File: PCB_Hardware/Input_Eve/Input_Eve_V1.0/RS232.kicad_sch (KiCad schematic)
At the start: 10 parts, among them U9 MAX3232

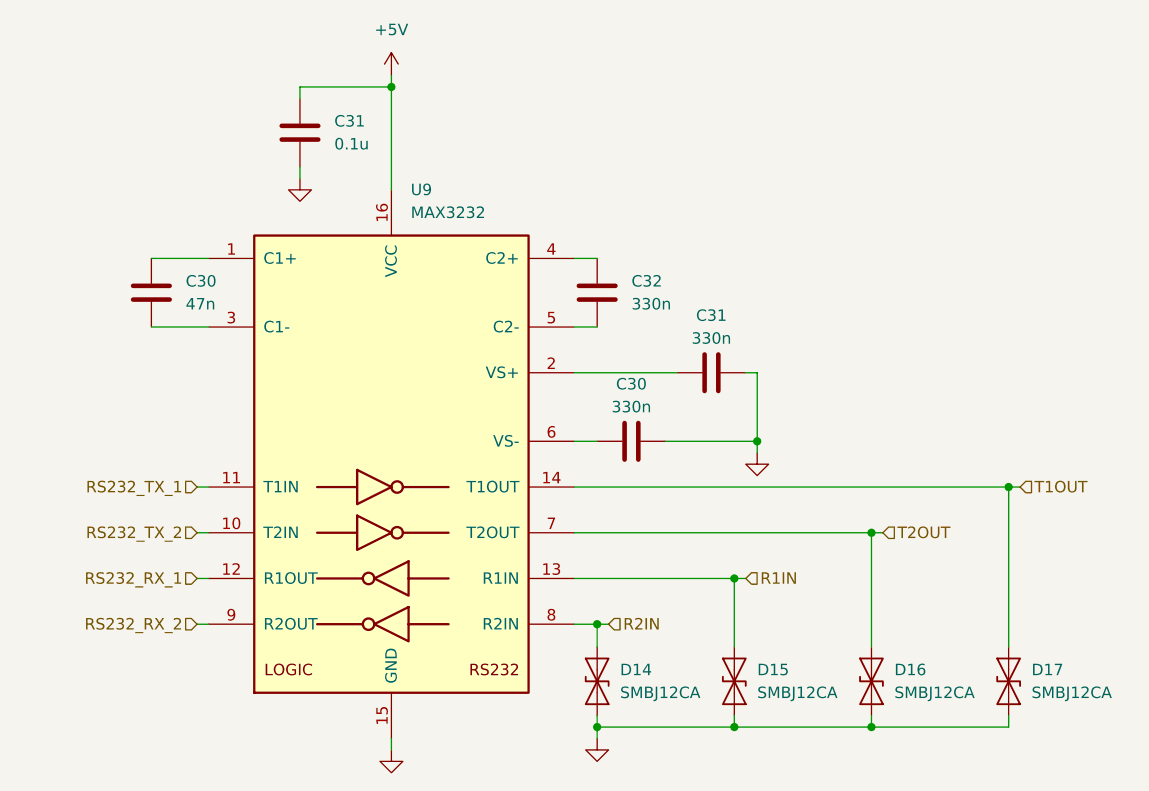
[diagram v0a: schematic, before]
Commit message: Update w new boards/firmware
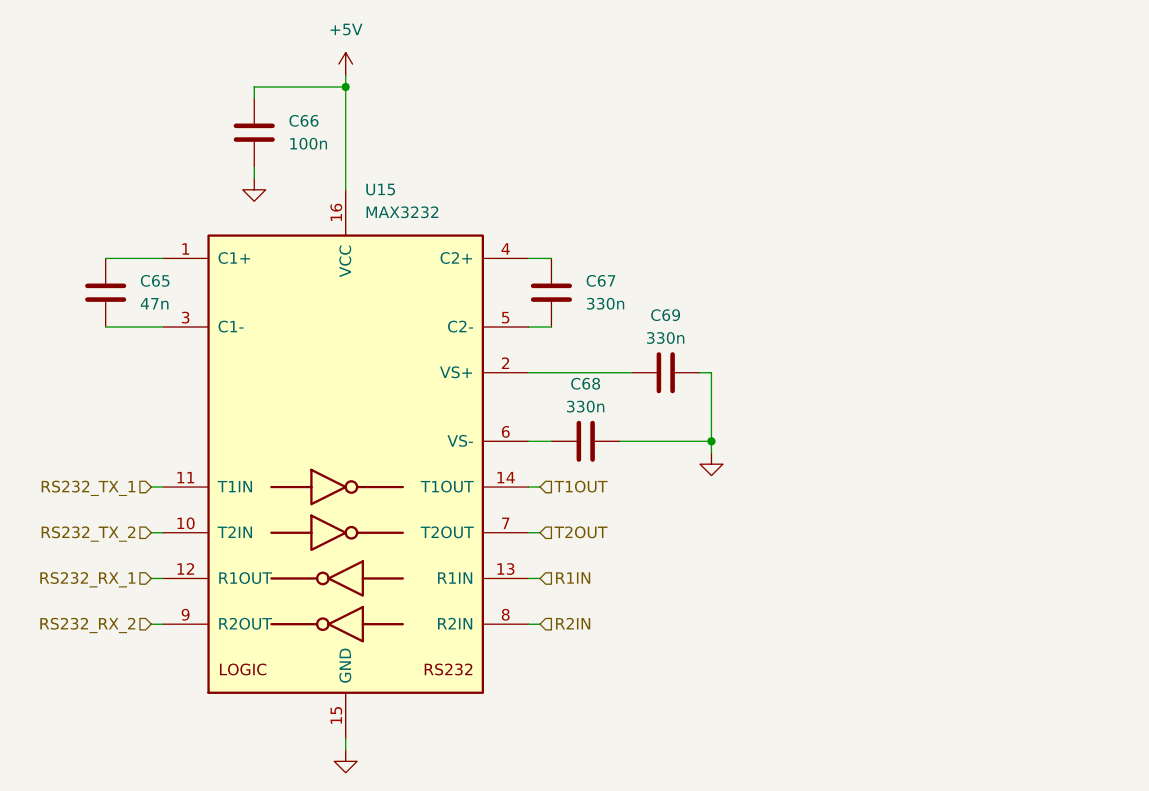
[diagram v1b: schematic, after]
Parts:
- removed C30: 47n, Capacitor_SMD:C_0402_1005Metric, symbol Device:C
- removed C30, C31, C32: 330n, Capacitor_SMD:C_0402_1005Metric, symbol Device:C
- removed C31: 0.1u, Capacitor_SMD:C_0402_1005Metric, symbol Device:C
- removed D14, D15, D16, D17: SMBJ12CA, Diode_SMD:D_SMA, symbol Diode:SMAJ6.0CA
- removed U9: MAX3232, symbol Interface_UART:MAX3232
- added C65: 47n, Capacitor_SMD:C_0402_1005Metric, symbol Device:C
- added C66: 100n, Capacitor_SMD:C_0402_1005Metric, symbol Device:C
- added C67, C68, C69: 330n, Capacitor_SMD:C_0402_1005Metric, symbol Device:C
- added U15: MAX3232, Package_SO:TSSOP-16_4.4x5mm_P0.65mm, symbol Interface_UART:MAX3232
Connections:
- net +5V: now also C66.1, U15.16 (VCC)
- net GND: now also C66.2, C68.2, C69.2, U15.15 (GND)
- net R1IN: now also U15.13 (R1IN)
- net R2IN: now also U15.8 (R2IN)
- net RS232_RX_1: now also U15.12 (R1OUT)
- net RS232_RX_2: now also U15.9 (R2OUT)
- net RS232_TX_1: now also U15.11 (T1IN)
- net RS232_TX_2: now also U15.10 (T2IN)
- net T1OUT: now also U15.14 (T1OUT)
- net T2OUT: now also U15.7 (T2OUT)
- new net: C69.1, U15.2 (VS+)
- new net: C67.1, U15.4 (C2+)
- new net: C67.2, U15.5 (C2-)
- new net: C65.1, U15.1 (C1+)
- new net: C65.2, U15.3 (C1-)
- new net: C68.1, U15.6 (VS-)
